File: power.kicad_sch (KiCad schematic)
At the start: 0 parts

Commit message: add Power Circuit
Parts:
- added C10, C11, C12, C5, C6, C7, C8, C9: C, symbol Device:C
- added C3: C_Polarized, symbol Device:C_Polarized
- added D3: CUHS20S30, SamacSys_Parts:CUHS20S40H3F, symbol Device:D_Schottky
- added D4: UDZV5.1B, Diode_SMD:D_SOD-323_HandSoldering, symbol Device:D_Zener
- added L1: L, symbol Device:L
- added Q1: AO3401A, Package_TO_SOT_SMD:SOT-23, symbol Transistor_FET:AO3401A
- added R10, R11, R12, R14, R4, R9: R, symbol Device:R
- added U1: TPS62933, Package_TO_SOT_SMD:SOT-583-8, symbol Regulator_Switching:TPS62933
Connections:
- new net: C11.1, R14.2
- new net: C11.2, L1.1, U1.5 (SW)
- new net: C12.1, U1.7 (SS)
- new net: D4.2 (A), Q1.1 (G), R4.1
- new net: R10.1, R9.2, U1.2 (EN)
- new net: R11.1, R12.1, U1.8 (FB)
- new net: R14.1, U1.6 (BST)
- new net +12V: C3.1, C5.1, C6.1, C7.1, D4.1 (K), Q1.2 (S), R9.1, U1.3 (VIN)
- new net +5V: C10.1, C8.1, C9.1, D3.1 (K), L1.2, R12.2
- new net +BATT: Q1.3 (D)
- new net GND: C12.2, C3.2, C5.2, C6.2, C7.2, R10.2, R11.2, R4.2, U1.4 (GND)
- new net VUSB: D3.2 (A)
- no-connect marks 0 -> 1

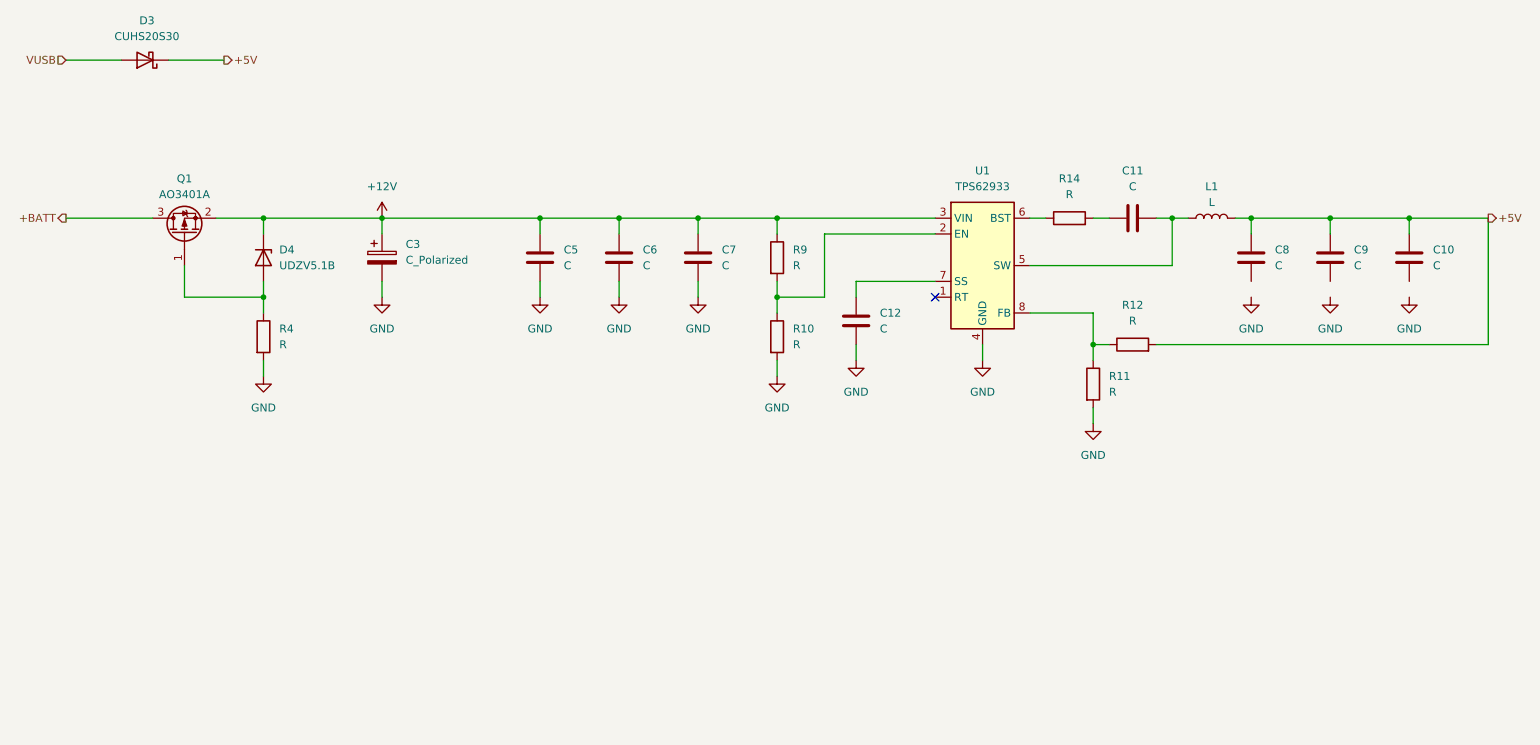
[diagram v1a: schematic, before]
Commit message: modify, add comment
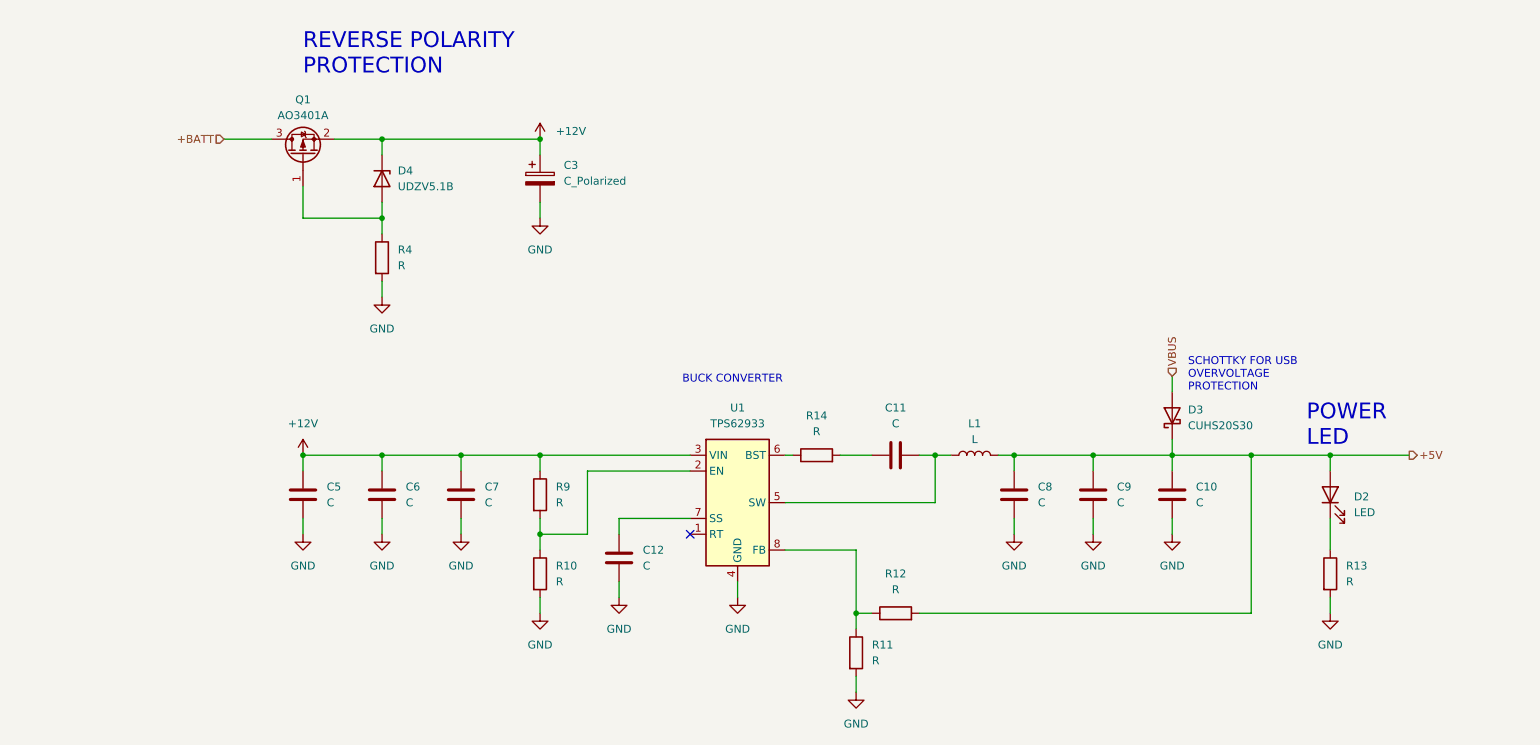
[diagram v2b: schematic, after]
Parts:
- added D2: LED, symbol Device:LED
- added R13: R, symbol Device:R
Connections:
- net +5V: now also D2.2 (A)
- net GND: now also C10.2, C8.2, C9.2, R13.2
- net VUSB renamed VBUS
- new net: D2.1 (K), R13.1
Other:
- note added: "BUCK CONVERTER"
- note added: "POWER LED"
- note added: "REVERSE POLARITY PROTECTION"
- note added: "SCHOTTKY FOR USB OVERVOLTAGE PROTECTION"
- moved on the sheet: C10, C11, C12, C3, C5, C6, C7, C8, C9, D3, D4, L1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

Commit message: add fuse, modify
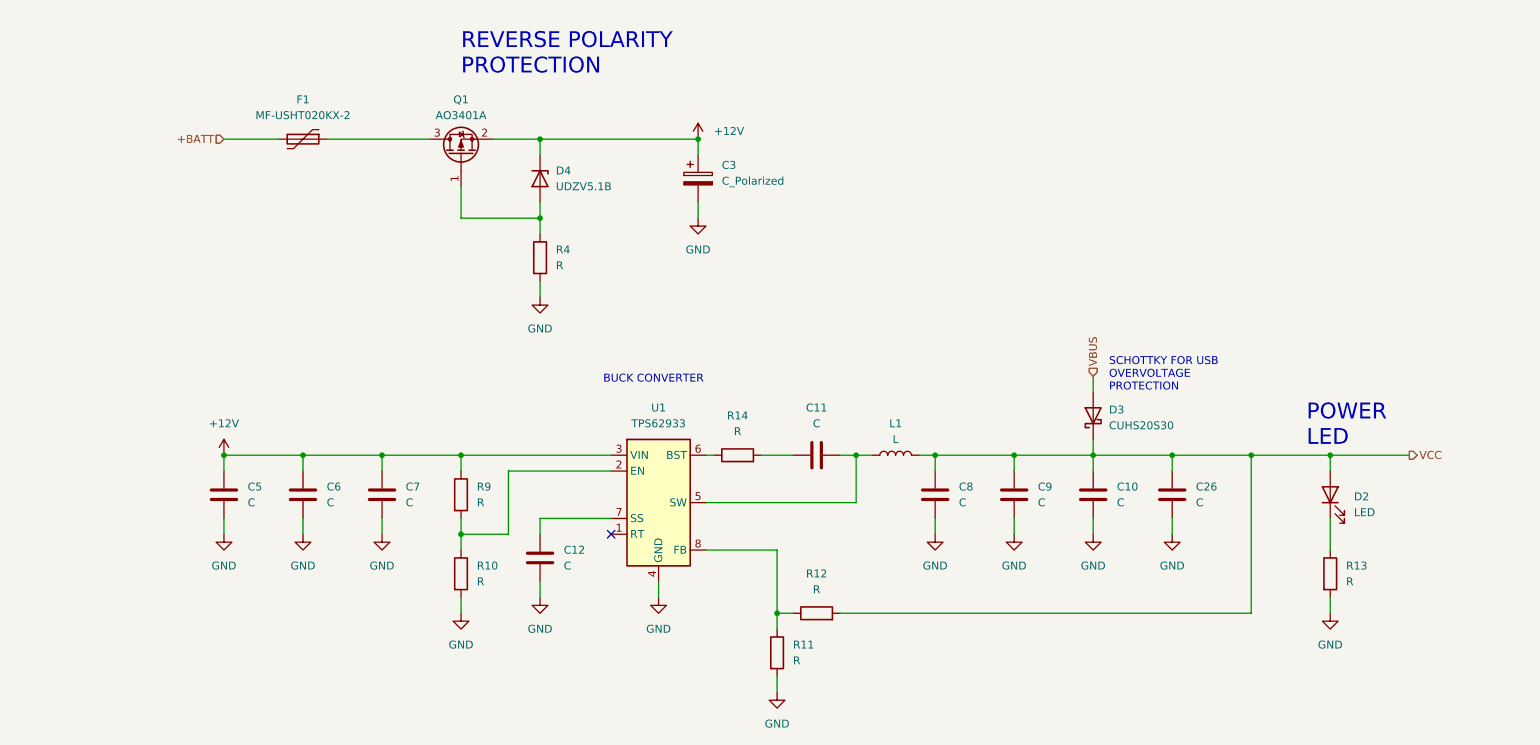
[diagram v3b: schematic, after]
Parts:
- added C26: C, symbol Device:C
- added F1: MF-USHT020KX-2, Fuse:Fuse_1210_3225Metric, symbol Device:Polyfuse
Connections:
- net +BATT: now also F1.2; no longer Q1.3 (D)
- net GND: now also C26.2
- net +5V renamed VCC
- net VCC: now also C26.1
- new net: F1.1, Q1.3 (D)
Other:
- moved on the sheet: C10, C11, C12, C3, C5, C6, C7, C8, C9, D3, D4, L1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
